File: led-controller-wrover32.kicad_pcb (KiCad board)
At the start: 4 copper layers, 36 x 40 mm, 132 parts, among them J101 Molex PicoBlade 4-pin, J102 Molex PicoBlade 6-pin, J103 STATUS OUT, J104 USB_B_Micro, J105 POWER IN, J106 Molex PicoBlade 6-pin, J107 5V_LOGIC, J201 12V_OUT, J301 Micro_SD_Card, J302 Molex PicoBlade 4-pin, J401 Fan PWM, J402 GPIO_CONN, Q101 UMH3N, Q102 BSS138, Q301 BSS138, Q401 SIL2301-TP, Q402 EM6K7T2R, SW301 KMR2, SW302 KMR2, U101 USBUF02W6, U102 ESP32-S3-WROOM-2-N32R8V, U103 NTS0104BQ,115, U104 TCA9406ZYPR, U202 MPM3810GQB-33, U203 TPS61089RNRR, U301 SSM2518CPZ, U401 SN74AUP1G08YZP, U402 BNO085, U403 PCA9575HF, Y401 OM-7604-C7

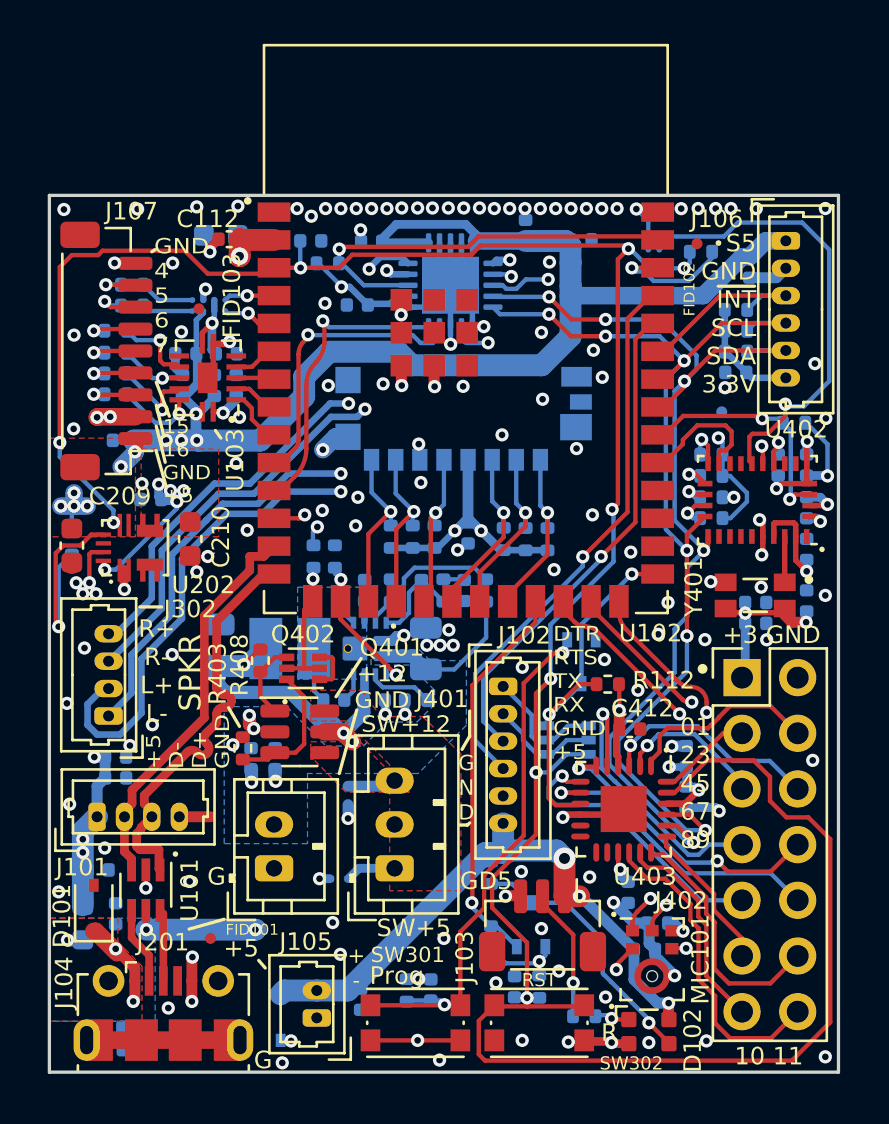
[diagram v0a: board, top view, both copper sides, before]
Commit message: Latest 4.0 settings for pcbway
Signed-off-by: Aaron Williams <aaron.w2@gmail.com>
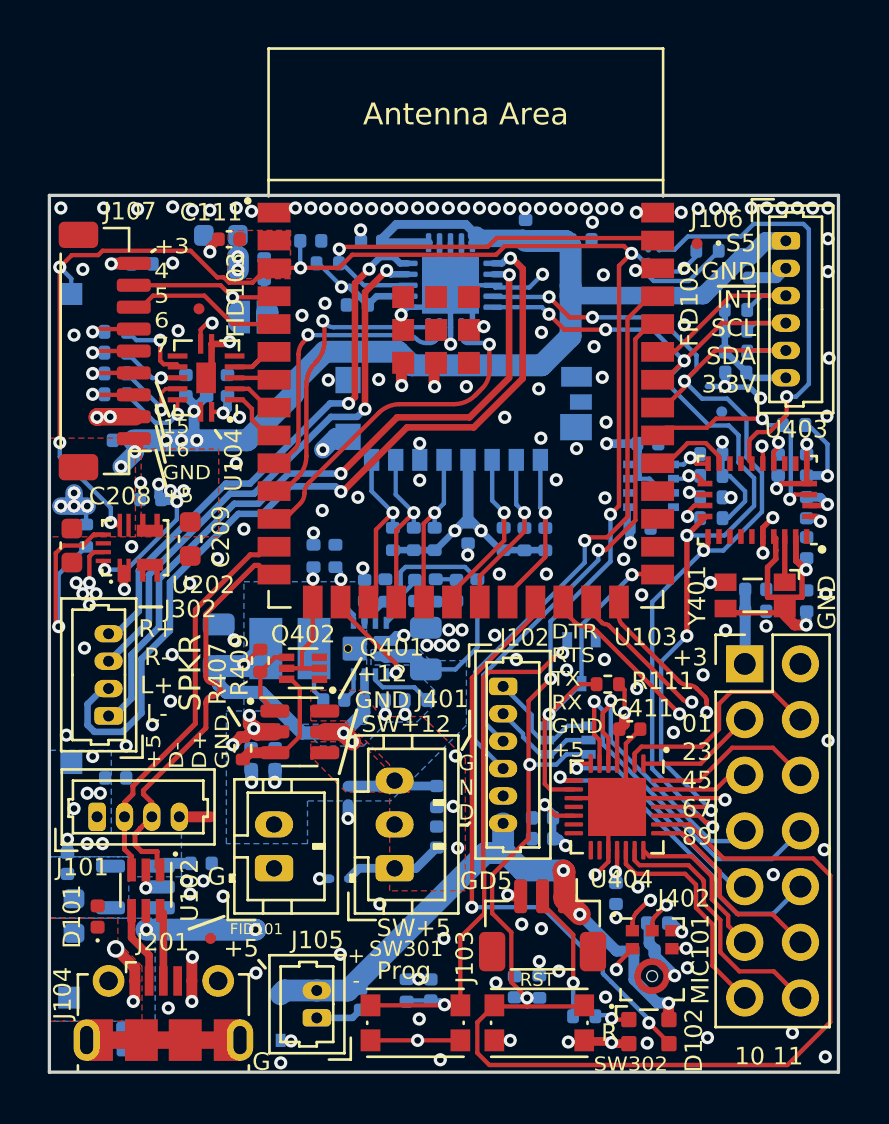
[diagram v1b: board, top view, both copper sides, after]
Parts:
- removed the C102 at (87.2, 64.4)
- removed the C103 at (63.0, 62.8)
- removed the C116 at (66.2, 37.2)
- removed Q102: BSS138, Package_TO_SOT_SMD:SOT-323_SC-70
- removed the R101 at (80.2, 63.9)
- removed the R102 at (80.2, 60.9)
- removed R113, R114: 33, Resistor_SMD:R_0402_1005Metric
- removed the R202 at (73.0, 46.5)
- removed the R405 at (90.2, 42.8)
- removed the U104 at (67.3, 35.0)
- removed the U403 at (86.2, 58.0)
- added C101: 1uF, Capacitor_SMD:C_0402_1005Metric, B.Cu at (87.1, 64.5)
- added C115: 1uF, Capacitor_SMD:C_0402_1005Metric, B.Cu at (69.8, 33.4)
- added C404: 0.1uF, Capacitor_SMD:C_0402_1005Metric, B.Cu at (87.3, 41.3)
- added C405: 0.1uF, Capacitor_SMD:C_0402_1005Metric, B.Cu at (87.0, 45.2)
- added C410: 1uF, Capacitor_SMD:C_0402_1005Metric, B.Cu at (77.7, 57.4)
- added C415: 1uF, Capacitor_SMD:C_0402_1005Metric, B.Cu at (77.7, 59.3)
- added JP101: IO4_IN_FILT, Jumper:SolderJumper-2_P1.3mm_Open_RoundedPad1.0x1.5mm, B.Cu at (69.3, 35.5)
- added R107: 10K, Resistor_SMD:R_0402_1005Metric, B.Cu at (73.0, 46.5)
- added R403: 2.2K, Resistor_SMD:R_0402_1005Metric, B.Cu at (90.2, 41.8)
- added TP101: TP +5_filtered, TestPoint:TestPoint_Pad_1.0x1.0mm, B.Cu at (61.0, 55.9)
- added TP102: TP +5_USB, TestPoint:TestPoint_Pad_1.0x1.0mm, B.Cu at (60.9, 66.6)
- added TP301: ~{RESET}, TestPoint:TestPoint_Pad_1.0x1.0mm, B.Cu at (61.0, 34.5)
- added U101: TPS2001DDBVX, Package_TO_SOT_SMD:SOT-23-5, B.Cu at (63.9, 61.5)
- added U402: BME280, Package_LGA:Bosch_LGA-8_2.5x2.5mm_P0.65mm_ClockwisePinNumbering, B.Cu at (87.5, 43.2)
- added U404: SX1509BIULTRT, Aaron:QFN-28-1EP_4x4mm_P0.4mm_EP2.65x2.65mm, F.Cu at (85.9, 57.9)
- C102: renamed from C104; value 0.1uF -> 1uF
- D101: value UDD32C12L01 -> TPD1E10B06DPYR; footprint Diode_SMD:D_SOD-323 -> Diode_SMD:D_0402_1005Metric
- D102: footprint marbastlib-various:LED_WS2812_2020 -> Aaron:LED_WS2812_2020
- R108: renamed from R109; value 4.7K -> 10K
- R404: value 4.7K -> 2.2K
- R407: renamed from R403; value 10K -> 110K
- R409: renamed from R408; value 10K -> 110K
- U103: renamed from U102; value ESP32-S3-WROOM-2-N32R8V -> ESP32-S3-WROOM-2-N32R8; footprint Aaron:ESP32-S3-WROOM-2-N32R8V -> Espressif:ESP32-S3-WROOM-2
- moved C413 7.55 mm to (82.5, 59.4), turned to 180 degrees
- moved C414 6.62 mm to (82.5, 58.4), turned to 180 degrees
- moved C103 6.22 mm to (66.9, 60.5)
- moved C114 5.62 mm to (64.2, 33.1)
- moved U103 2.95 mm to (79.0, 39.0)
- moved C102 1.43 mm to (60.8, 60.5), turned to 90 degrees
- moved R404 0.97 mm to (90.2, 42.8)
- moved R206 0.74 mm to (61.7, 45.5)
- moved J402 0.64 mm to (91.7, 51.4)
- moved C416 0.60 mm to (92.2, 48.0)
- moved C412 0.55 mm to (85.8, 61.9)
- moved C417 0.55 mm to (92.2, 49.0)
- moved FB101 0.50 mm to (61.1, 62.9)
- moved D101 0.41 mm to (62.2, 62.9)
- moved C107 0.40 mm to (68.1, 38.7)
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- renumbered C101 to C103, C105 to C104, C106 to C105, C107 to C106, C108 to C107, C109 to C108, C110 to C109, C111 to C110, C112 to C111, C113 to C112, C114 to C113, C115 to C114, C117 to C116, C118 to C117, C212 to C201, C214 to C202, C215 to C203, C213 to C204, C216 to C205, C217 to C206, C218 to C207, C209 to C208, C210 to C209, C211 to C210, C404 to C406, C405 to C408, C406 to C409, C412 to C411, C413 to C412, C410 to C413, C411 to C414, C408 to C416, C409 to C417, L202 to L201, R103 to R101, R104 to R102, R105 to R103, R106 to R104, R107 to R105, R108 to R106, R110 to R109, R111 to R110, R112 to R111, R207 to R201, R208 to R202, R210 to R203, R209 to R204, R211 to R205, R407 to R405, R409 to R406, R406 to R408, U101 to U102, U103 to U104, U203 to U201, U402 to U403
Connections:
- net /Motion and GPIO/SW_5V_IO1 renamed /Motion and GPIO/SW_5V
- net Net-(U401-PadC2) renamed /Motion and GPIO/~{BNO085_RST}
- C102 pad 1: +5V -> /FVUSB
- D102 pad 3: /STS_5V -> /STATUS_LED
- FB101 pad 2: +5V -> /FVUSB
- J107 pad 7: /IO5_H -> /IO5
- J107 pad 8: /IO4_H -> /IO4
- J107 pad 9: GND -> +3V3
- J402 pad 11: /Motion and GPIO/P1_0 -> /Motion and GPIO/P0_14
- J402 pad 12: /Motion and GPIO/P1_1 -> /Motion and GPIO/P0_15
- J402 pad 13: /Motion and GPIO/P1_2 -> /Motion and GPIO/P0_12
- J402 pad 14: /Motion and GPIO/P1_3 -> /Motion and GPIO/P0_13
- J402 pad 3: /Motion and GPIO/P0_0 -> /Motion and GPIO/P0_2
- J402 pad 4: /Motion and GPIO/P0_1 -> /Motion and GPIO/P0_3
- J402 pad 5: /Motion and GPIO/P0_2 -> /Motion and GPIO/P0_0
- J402 pad 6: /Motion and GPIO/P0_3 -> /Motion and GPIO/P0_1
- R404 pad 1: /Motion and GPIO/H_SCL -> /Motion and GPIO/S_SDA
- U301 pad 3: +3V3 -> GND
- U403 pad 15: /Motion and GPIO/H_SCL -> /Motion and GPIO/S_SCL
- U403 pad 16: /Motion and GPIO/H_SDA -> /Motion and GPIO/S_SDA
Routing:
- net /Motion and GPIO/P1_3: track 14.5 -> 0.00 mm
- net +5V: track 114.0 -> 101.5 mm, vias 19 -> 22
- net /Motion and GPIO/P0_13: track 0.00 -> 12.1 mm
- net /STS_5V: track 12.1 -> 0.00 mm, vias 1 -> 0
- net /Motion and GPIO/P1_1: track 11.3 -> 0.00 mm
- net /Motion and GPIO/P0_12: track 0.00 -> 10.3 mm
- net GND: track 59.9 -> 69.8 mm, vias 150 -> 183
- net /Motion and GPIO/P1_2: track 9.71 -> 0.00 mm
- net /Motion and GPIO/P0_15: track 0.00 -> 9.11 mm
- net /STATUS_LED: track 17.6 -> 26.3 mm, vias 1 -> 2
- net /Motion and GPIO/P0_14: track 0.00 -> 7.24 mm
- net /Motion and GPIO/P1_0: track 6.16 -> 0.00 mm
- net /IO4: track 2.31 -> 7.19 mm
- net /IO5: track 2.46 -> 6.80 mm, vias 1 -> 0
- net +3V3: track 90.9 -> 94.3 mm, vias 31 -> 33
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- added copper zone on B.Cu, net +5V
- added copper zone on B.Cu, net /FVUSB
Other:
- board text added: "+3 4 5 6 7"
- board text added: "DT RTS TX RX GN +5"
- board text added: "GND"
- board text added: "GND SW 5"
- board text added: "JP101 filter IO4"
- board text added: "SW 12"
- board text added: "~{RESET}"
- board text removed: "+3 GND"
- board text removed: "D R TX RX GND +5V"
- board text removed: "GND 4 5 6 7"
- board text removed: "GND SW5"
